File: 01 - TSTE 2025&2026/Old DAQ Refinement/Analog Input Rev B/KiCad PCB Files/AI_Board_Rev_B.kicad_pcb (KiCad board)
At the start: 2 copper layers, 130 x 165 mm, 54 parts, among them J1 DC37_Socket_MountingHoles, J10 AI4 M12, J11 AI4 XT30, J12 AI5 M12, J13 AI5 XT30, J14 AI6 M12, J15 AI6 XT30, J16 AI7 M12, J17 AI7 XT30, J18 AI8 M12, J19 AI8 XT30, J2 AI0 M12, J20 AI9 M12, J21 AI9 XT30, J22 AI10 M12, J23 AI10 XT30, J24 AI11 M12, J25 AI11 XT30, J26 AI12 M12, J27 AI12 XT30, J28 AI13 M12, J29 AI13 XT30, J3 AI0 XT30, J30 AI14 M12, J31 AI14 XT30, J32 AI15 M12, J33 AI15 XT30, J4 AI1 M12, J5 AI1 XT30, J6 AI2 M12, J7 AI2 XT30, J8 AI3 M12, J9 AI3 XT30, M3 MountingHole_3.2mm_M3

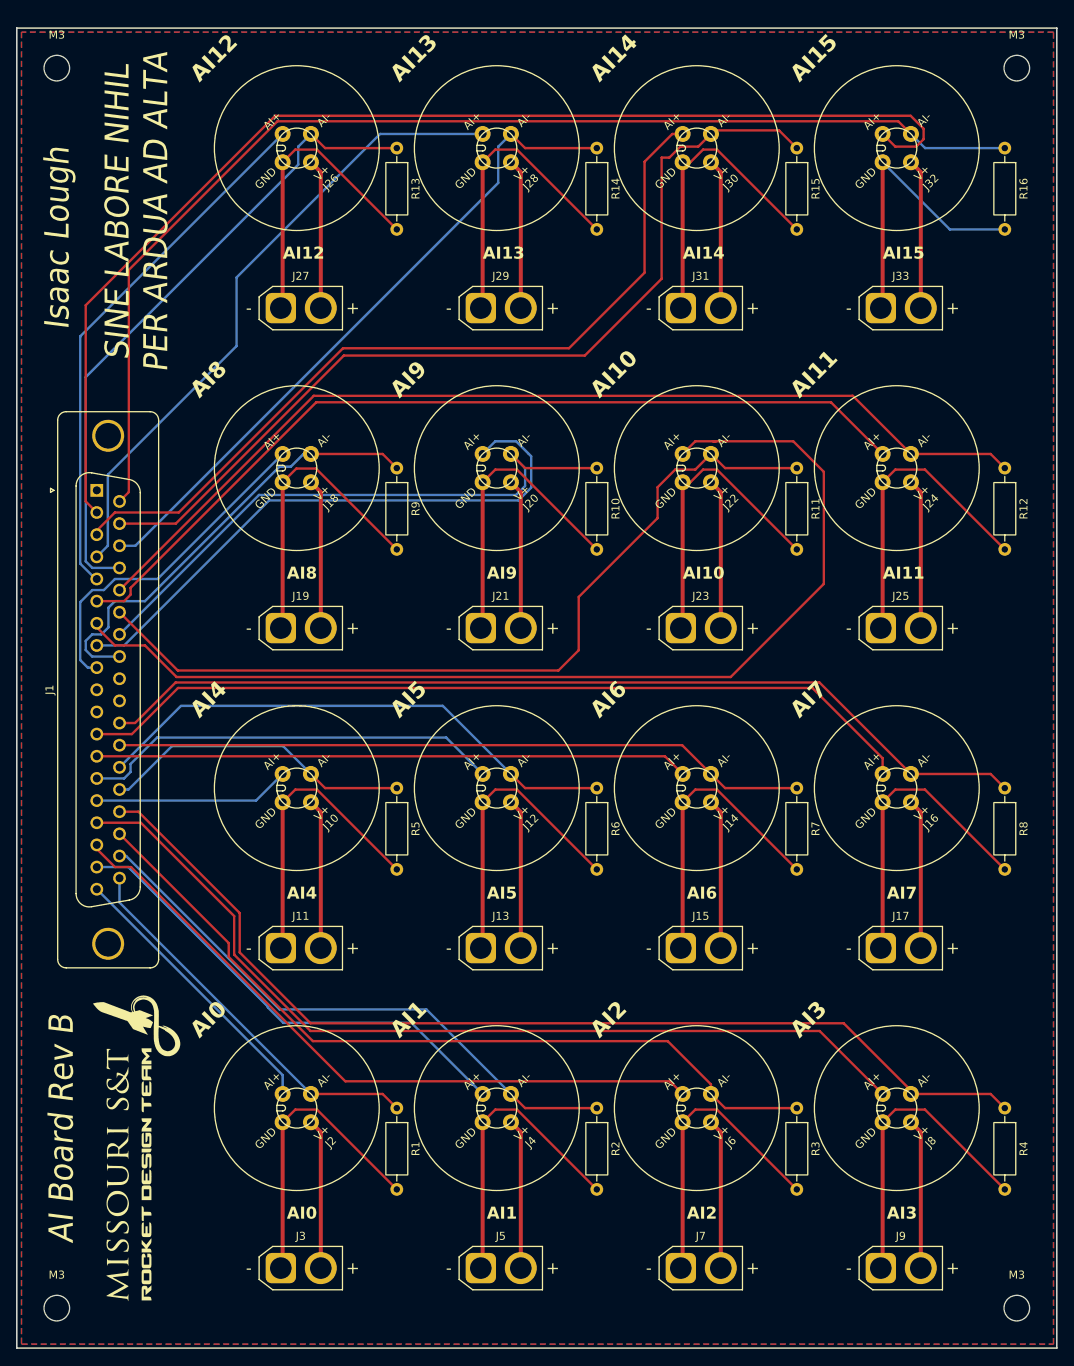
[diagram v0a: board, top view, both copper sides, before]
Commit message: Final Files
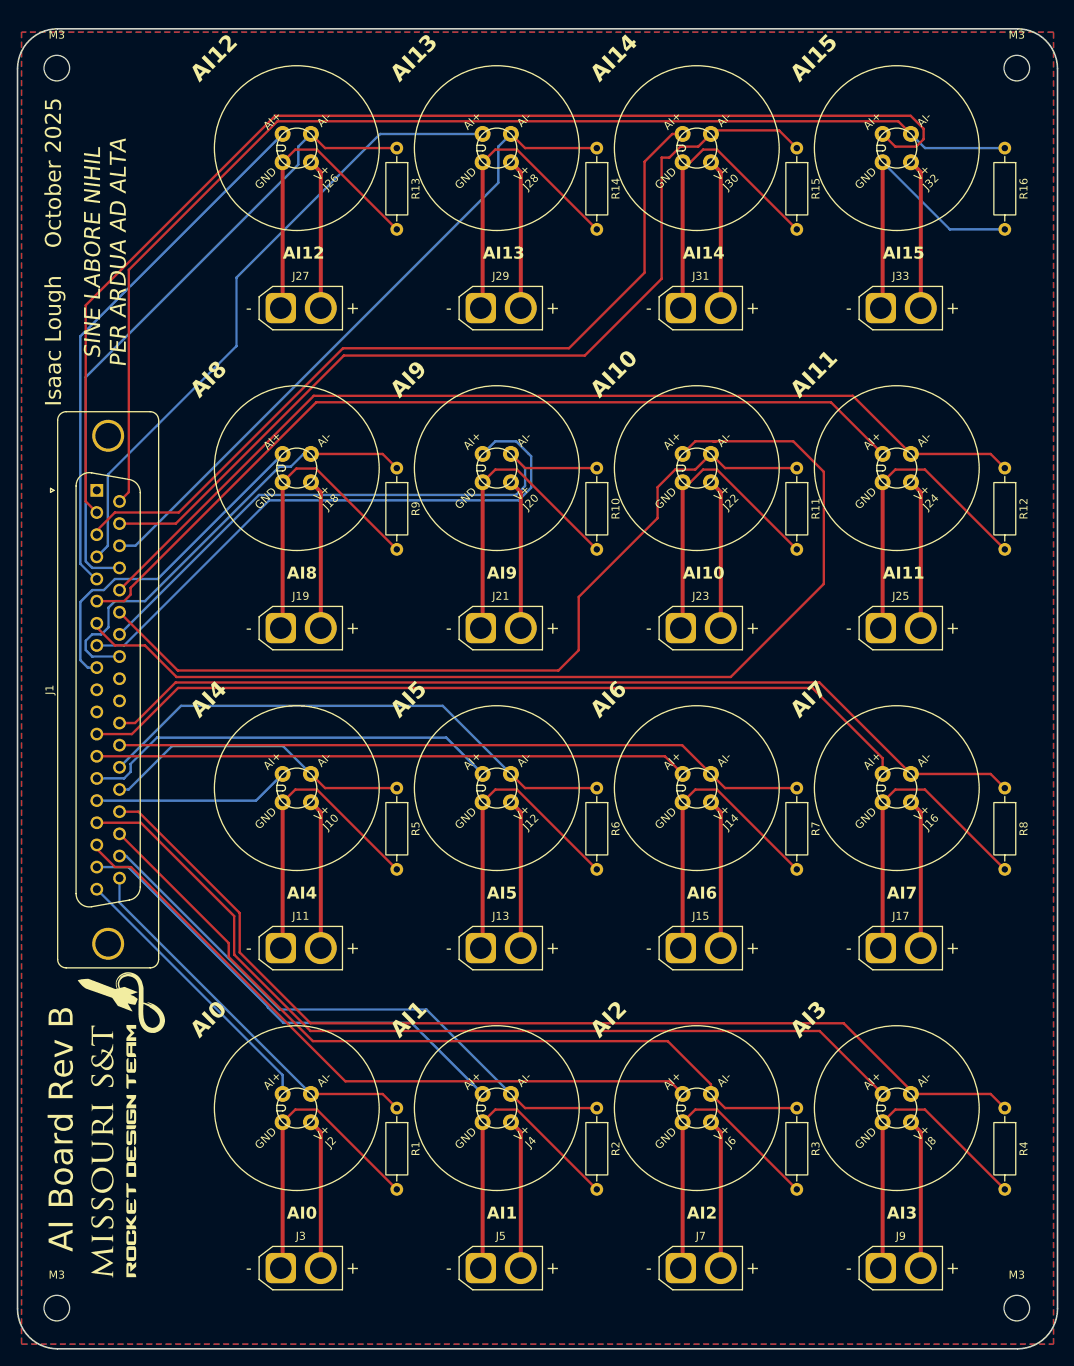
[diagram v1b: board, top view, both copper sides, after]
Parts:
- moved G*** 3.48 mm to (28.1, 152.1)
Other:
- outline, holes or cut-outs redrawn
- board text added: "October 2025"
